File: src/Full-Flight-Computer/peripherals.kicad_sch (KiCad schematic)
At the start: 40 parts, among them P1 1984659, P4 1546551-4, P4 1984659, P6 USB, Q1 QS5U17TR, Q2 2N7002W-7-F, Q3 2N7002W-7-F, Q4 QS5U17TR, Q5 2N7002W-7-F, Q6 2N7002W-7-F, U7 SST25VF040B-50-4I-S2AE-T, U8 CP2102-GMR(QFN28)

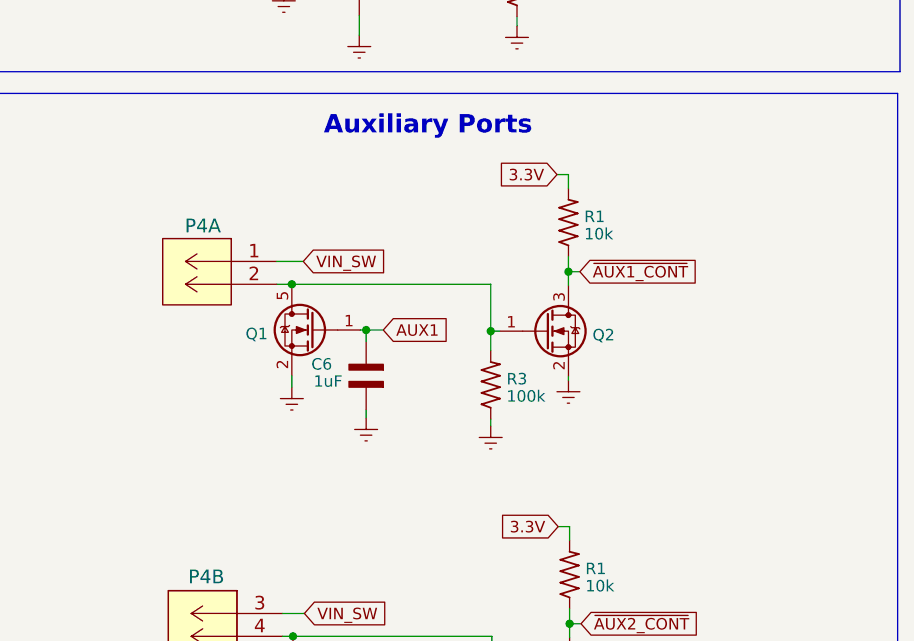
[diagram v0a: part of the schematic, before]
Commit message: completed initial layout
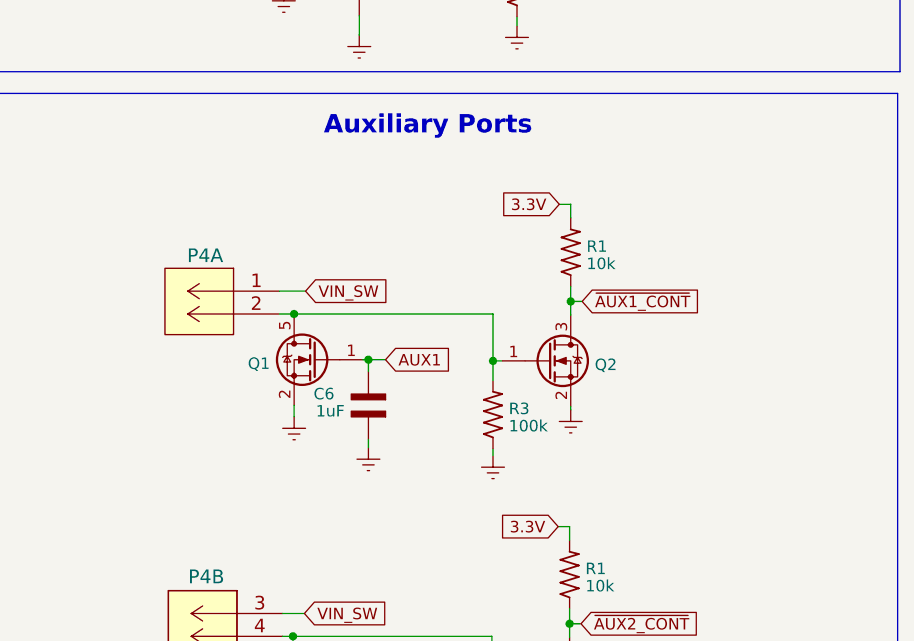
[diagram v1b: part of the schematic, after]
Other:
- moved on the sheet: C6, P4A, Q1, Q2, R1, R3
